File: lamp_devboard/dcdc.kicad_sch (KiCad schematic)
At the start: 10 parts, among them U601 TPS63060

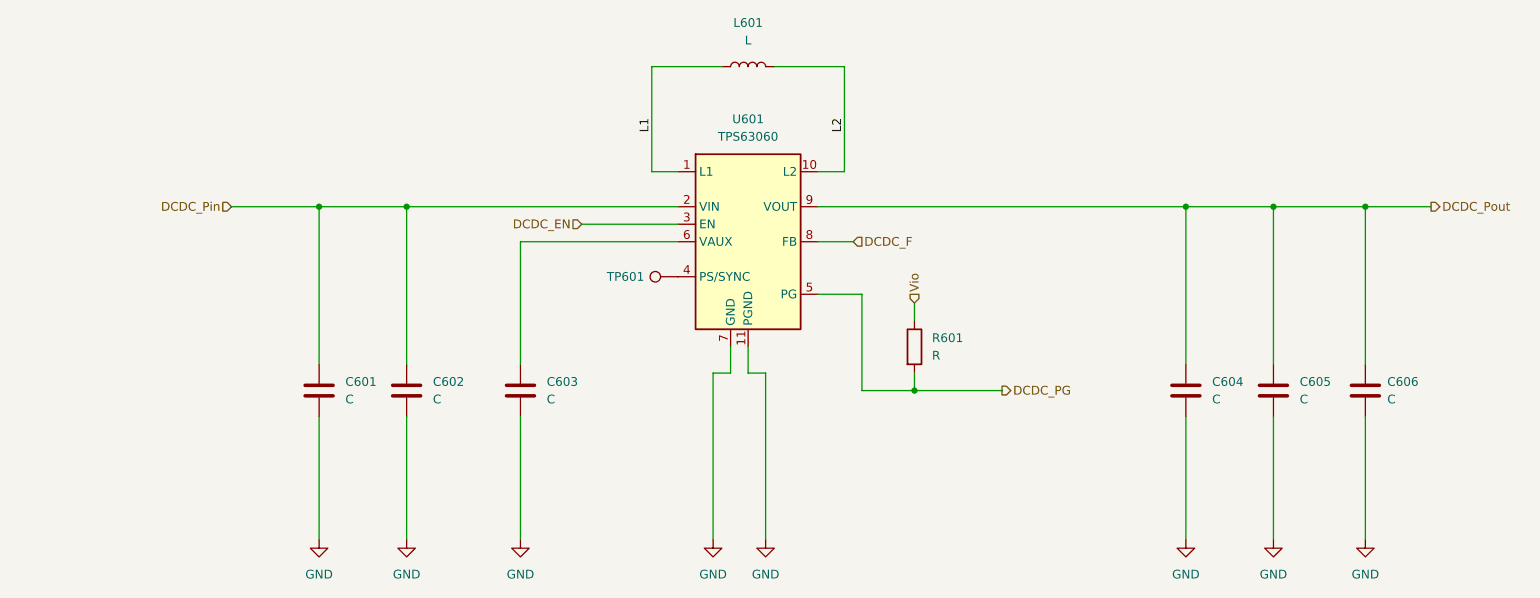
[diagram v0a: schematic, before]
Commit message: first version of the pcb board
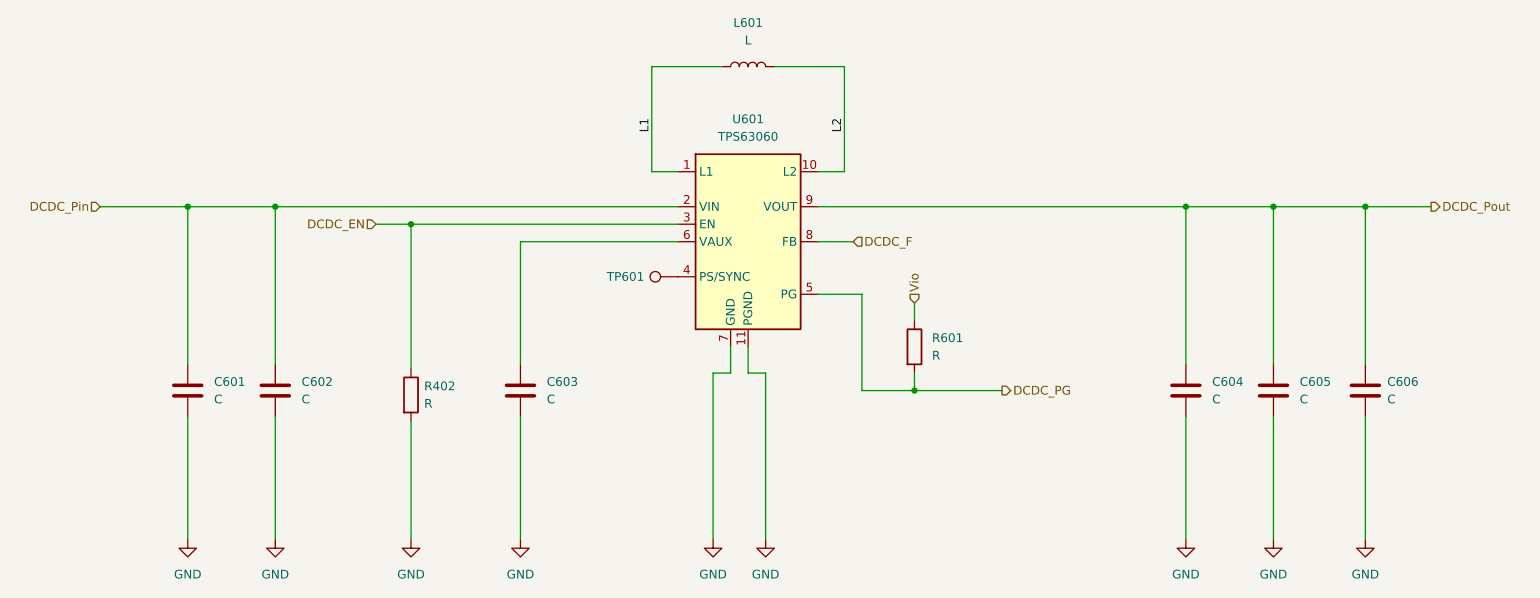
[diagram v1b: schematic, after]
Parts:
- added R402: R, Resistor_SMD:R_0603_1608Metric_Pad0.98x0.95mm_HandSolder, symbol Device:R
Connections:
- net DCDC_EN: now also R402.1
- net GND: now also R402.2
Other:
- moved on the sheet: C601, C602
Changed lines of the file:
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@@
   (junction (at 201.93 90.17) (diameter 0) (color 0 0 0 0)
   )
+  (junction (at 76.835 92.71) (diameter 0) (color 0 0 0 0)
+  )
   (junction (at 149.86 116.84) (diameter 0) (color 0 0 0 0)
   )
@@
   (junction (at 189.23 90.17) (diameter 0) (color 0 0 0 0)
   )
-  (junction (at 63.5 90.17) (diameter 0) (color 0 0 0 0)
-  )
-  (junction (at 76.2 90.17) (diameter 0) (color 0 0 0 0)
+  (junction (at 44.45 90.17) (diameter 0) (color 0 0 0 0)
+  )
+  (junction (at 57.15 90.17) (diameter 0) (color 0 0 0 0)
   )
   (wire (pts (xy 201.93 90.17) (xy 201.93 113.03))
@@
     (stroke (width 0) (type default) (color 0 0 0 0))
   )
-  (wire (pts (xy 50.8 90.17) (xy 63.5 90.17))
-    (stroke (width 0) (type default) (color 0 0 0 0))
-  )
-  (wire (pts (xy 76.2 120.65) (xy 76.2 138.43))
+  (wire (pts (xy 31.75 90.17) (xy 44.45 90.17))
+    (stroke (width 0) (type default) (color 0 0 0 0))
+  )
+  (wire (pts (xy 57.15 120.65) (xy 57.15 138.43))
     (stroke (width 0) (type default) (color 0 0 0 0))
   )
@@
     (stroke (width 0) (type default) (color 0 0 0 0))
   )
-  (wire (pts (xy 76.2 113.03) (xy 76.2 90.17))
+  (wire (pts (xy 57.15 113.03) (xy 57.15 90.17))
     (stroke (width 0) (type default) (color 0 0 0 0))
   )
@@
     (stroke (width 0) (type default) (color 0 0 0 0))
   )
-  (wire (pts (xy 101.6 92.71) (xy 115.57 92.71))
-    (stroke (width 0) (type default) (color 0 0 0 0))
-  )
-  (wire (pts (xy 76.2 90.17) (xy 115.57 90.17))
+  (wire (pts (xy 76.835 138.43) (xy 76.835 121.285))
+    (stroke (width 0) (type default) (color 0 0 0 0))
+  )
+  (wire (pts (xy 71.755 92.71) (xy 76.835 92.71))
+    (stroke (width 0) (type default) (color 0 0 0 0))
+  )
+  (wire (pts (xy 57.15 90.17) (xy 115.57 90.17))
     (stroke (width 0) (type default) (color 0 0 0 0))
   )
@@
     (stroke (width 0) (type default) (color 0 0 0 0))
   )
-  (wire (pts (xy 63.5 113.03) (xy 63.5 90.17))
+  (wire (pts (xy 44.45 113.03) (xy 44.45 90.17))
     (stroke (width 0) (type default) (color 0 0 0 0))
   )
@@
     (stroke (width 0) (type default) (color 0 0 0 0))
   )
-  (wire (pts (xy 63.5 90.17) (xy 76.2 90.17))
+  (wire (pts (xy 44.45 90.17) (xy 57.15 90.17))
+    (stroke (width 0) (type default) (color 0 0 0 0))
+  )
+  (wire (pts (xy 76.835 92.71) (xy 76.835 113.665))
     (stroke (width 0) (type default) (color 0 0 0 0))
   )
@@
     (stroke (width 0) (type default) (color 0 0 0 0))
   )
-  (wire (pts (xy 63.5 120.65) (xy 63.5 138.43))
+  (wire (pts (xy 44.45 120.65) (xy 44.45 138.43))
     (stroke (width 0) (type default) (color 0 0 0 0))
   )
@@
   )
   (wire (pts (xy 215.265 113.03) (xy 215.265 90.17))
+    (stroke (width 0) (type default) (color 0 0 0 0))
+  )
+  (wire (pts (xy 76.835 92.71) (xy 115.57 92.71))
     (stroke (width 0) (type default) (color 0 0 0 0))
   )
@@
     (effects (font (size 1.27 1.27)) (justify left))
   )
-  (hierarchical_label "DCDC_EN" (shape input) (at 101.6 92.71 180)
+  (hierarchical_label "DCDC_EN" (shape input) (at 71.755 92.71 180)
     (effects (font (size 1.27 1.27)) (justify right))
   )
@@
     (effects (font (size 1.27 1.27)) (justify left))
   )
-  (hierarchical_label "DCDC_Pin" (shape input) (at 50.8 90.17 180)
+  (hierarchical_label "DCDC_Pin" (shape input) (at 31.75 90.17 180)
     (effects (font (size 1.27 1.27)) (justify right))
   )
@@
     (pin "1")
   )
-  (symbol (lib_id "power:GND") (at 63.5 138.43 0) (unit 1)
-    (in_bom yes) (on_board yes) (fields_autoplaced)
-    (property "Reference" "#PWR0132" (id 0) (at 63.5 144.78 0)
-      (effects (font (size 1.27 1.27)) hide)
-    )
-    (property "Value" "GND" (id 1) (at 63.5 143.51 0))
-    (property "Footprint" "" (id 2) (at 63.5 138.43 0)
-      (effects (font (size 1.27 1.27)) hide)
-    )
-    (property "Datasheet" "" (id 3) (at 63.5 138.43 0)
-      (effects (font (size 1.27 1.27)) hide)
-    )
-    (pin "1")
-  )
-  (symbol (lib_id "power:GND") (at 76.2 138.43 0) (unit 1)
-    (in_bom yes) (on_board yes) (fields_autoplaced)
-    (property "Reference" "#PWR0131" (id 0) (at 76.2 144.78 0)
-      (effects (font (size 1.27 1.27)) hide)
-    )
-    (property "Value" "GND" (id 1) (at 76.2 143.51 0))
-    (property "Footprint" "" (id 2) (at 76.2 138.43 0)
-      (effects (font (size 1.27 1.27)) hide)
-    )
-    (property "Datasheet" "" (id 3) (at 76.2 138.43 0)
+  (symbol (lib_id "power:GND") (at 44.45 138.43 0) (unit 1)
+    (in_bom yes) (on_board yes) (fields_autoplaced)
+    (property "Reference" "#PWR0132" (id 0) (at 44.45 144.78 0)
+      (effects (font (size 1.27 1.27)) hide)
+    )
+    (property "Value" "GND" (id 1) (at 44.45 143.51 0))
+    (property "Footprint" "" (id 2) (at 44.45 138.43 0)
+      (effects (font (size 1.27 1.27)) hide)
+    )
+    (property "Datasheet" "" (id 3) (at 44.45 138.43 0)
+      (effects (font (size 1.27 1.27)) hide)
+    )
+    (pin "1")
+  )
+  (symbol (lib_id "power:GND") (at 57.15 138.43 0) (unit 1)
+    (in_bom yes) (on_board yes) (fields_autoplaced)
+    (property "Reference" "#PWR0131" (id 0) (at 57.15 144.78 0)
+      (effects (font (size 1.27 1.27)) hide)
+    )
+    (property "Value" "GND" (id 1) (at 57.15 143.51 0))
+    (property "Footprint" "" (id 2) (at 57.15 138.43 0)
+      (effects (font (size 1.27 1.27)) hide)
+    )
+    (property "Datasheet" "" (id 3) (at 57.15 138.43 0)
       (effects (font (size 1.27 1.27)) hide)
     )
@@
     (pin "1")
   )
-  (symbol (lib_id "Device:C") (at 63.5 116.84 0) (unit 1)
-    (in_bom yes) (on_board yes) (fields_autoplaced)
-    (property "Reference" "C601" (id 0) (at 67.31 115.5699 0)
-      (effects (font (size 1.27 1.27)) (justify left))
-    )
-    (property "Value" "C" (id 1) (at 67.31 118.1099 0)
-      (effects (font (size 1.27 1.27)) (justify left))
-    )
-    (property "Footprint" "Capacitor_SMD:C_1206_3216Metric_Pad1.33x1.80mm_HandSolder" (id 2) (at 64.4652 120.65 0)
-      (effects (font (size 1.27 1.27)) hide)
-    )
-    (property "Datasheet" "~" (id 3) (at 63.5 116.84 0)
+  (symbol (lib_id "Device:C") (at 44.45 116.84 0) (unit 1)
+    (in_bom yes) (on_board yes) (fields_autoplaced)
+    (property "Reference" "C601" (id 0) (at 48.26 115.5699 0)
+      (effects (font (size 1.27 1.27)) (justify left))
+    )
+    (property "Value" "C" (id 1) (at 48.26 118.1099 0)
+      (effects (font (size 1.27 1.27)) (justify left))
+    )
+    (property "Footprint" "Capacitor_SMD:C_1206_3216Metric_Pad1.33x1.80mm_HandSolder" (id 2) (at 45.4152 120.65 0)
+      (effects (font (size 1.27 1.27)) hide)
+    )
+    (property "Datasheet" "~" (id 3) (at 44.45 116.84 0)
       (effects (font (size 1.27 1.27)) hide)
     )
@@
     (pin "1")
   )
+  (symbol (lib_id "Device:R") (at 76.835 117.475 0) (unit 1)
+    (in_bom yes) (on_board yes) (fields_autoplaced)
+    (property "Reference" "R402" (id 0) (at 78.74 116.2049 0)
+      (effects (font (size 1.27 1.27)) (justify left))
+    )
+    (property "Value" "R" (id 1) (at 78.74 118.7449 0)
+      (effects (font (size 1.27 1.27)) (justify left))
+    )
+    (property "Footprint" "Resistor_SMD:R_0603_1608Metric_Pad0.98x0.95mm_HandSolder" (id 2) (at 75.057 117.475 90)
+      (effects (font (size 1.27 1.27)) hide)
+    )
+    (property "Datasheet" "~" (id 3) (at 76.835 117.475 0)
+      (effects (font (size 1.27 1.27)) hide)
+    )
+    (pin "1")
+    (pin "2")
+  )
   (symbol (lib_id "Device:C") (at 92.71 116.84 0) (unit 1)
     (in_bom yes) (on_board yes) (fields_autoplaced)
@@
     (pin "2")
   )
-  (symbol (lib_id "Device:C") (at 76.2 116.84 0) (unit 1)
-    (in_bom yes) (on_board yes) (fields_autoplaced)
-    (property "Reference" "C602" (id 0) (at 80.01 115.5699 0)
-      (effects (font (size 1.27 1.27)) (justify left))
-    )
-    (property "Value" "C" (id 1) (at 80.01 118.1099 0)
-      (effects (font (size 1.27 1.27)) (justify left))
-    )
-    (property "Footprint" "Capacitor_SMD:C_0603_1608Metric_Pad1.08x0.95mm_HandSolder" (id 2) (at 77.1652 120.65 0)
-      (effects (font (size 1.27 1.27)) hide)
-    )
-    (property "Datasheet" "~" (id 3) (at 76.2 116.84 0)
+  (symbol (lib_id "Device:C") (at 57.15 116.84 0) (unit 1)
+    (in_bom yes) (on_board yes) (fields_autoplaced)
+    (property "Reference" "C602" (id 0) (at 60.96 115.5699 0)
+      (effects (font (size 1.27 1.27)) (justify left))
+    )
+    (property "Value" "C" (id 1) (at 60.96 118.1099 0)
+      (effects (font (size 1.27 1.27)) (justify left))
+    )
+    (property "Footprint" "Capacitor_SMD:C_0603_1608Metric_Pad1.08x0.95mm_HandSolder" (id 2) (at 58.1152 120.65 0)
+      (effects (font (size 1.27 1.27)) hide)
+    )
+    (property "Datasheet" "~" (id 3) (at 57.15 116.84 0)
       (effects (font (size 1.27 1.27)) hide)
     )
@@
     (pin "2")
   )
+  (symbol (lib_id "power:GND") (at 76.835 138.43 0) (unit 1)
+    (in_bom yes) (on_board yes) (fields_autoplaced)
+    (property "Reference" "#PWR0151" (id 0) (at 76.835 144.78 0)
+      (effects (font (size 1.27 1.27)) hide)
+    )
+    (property "Value" "GND" (id 1) (at 76.835 143.51 0))
+    (property "Footprint" "" (id 2) (at 76.835 138.43 0)
+      (effects (font (size 1.27 1.27)) hide)
+    )
+    (property "Datasheet" "" (id 3) (at 76.835 138.43 0)
+      (effects (font (size 1.27 1.27)) hide)
+    )
+    (pin "1")
+  )
   (symbol (lib_id "power:GND") (at 215.265 138.43 0) (unit 1)
